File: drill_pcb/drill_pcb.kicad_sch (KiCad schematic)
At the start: 38 parts, among them SW1 RPi reset, U1 PCA9306, U2 Pico, U3 L7805, U4 IFX007T, U5 IFX007T, U6 ACS712xLCTR-20A

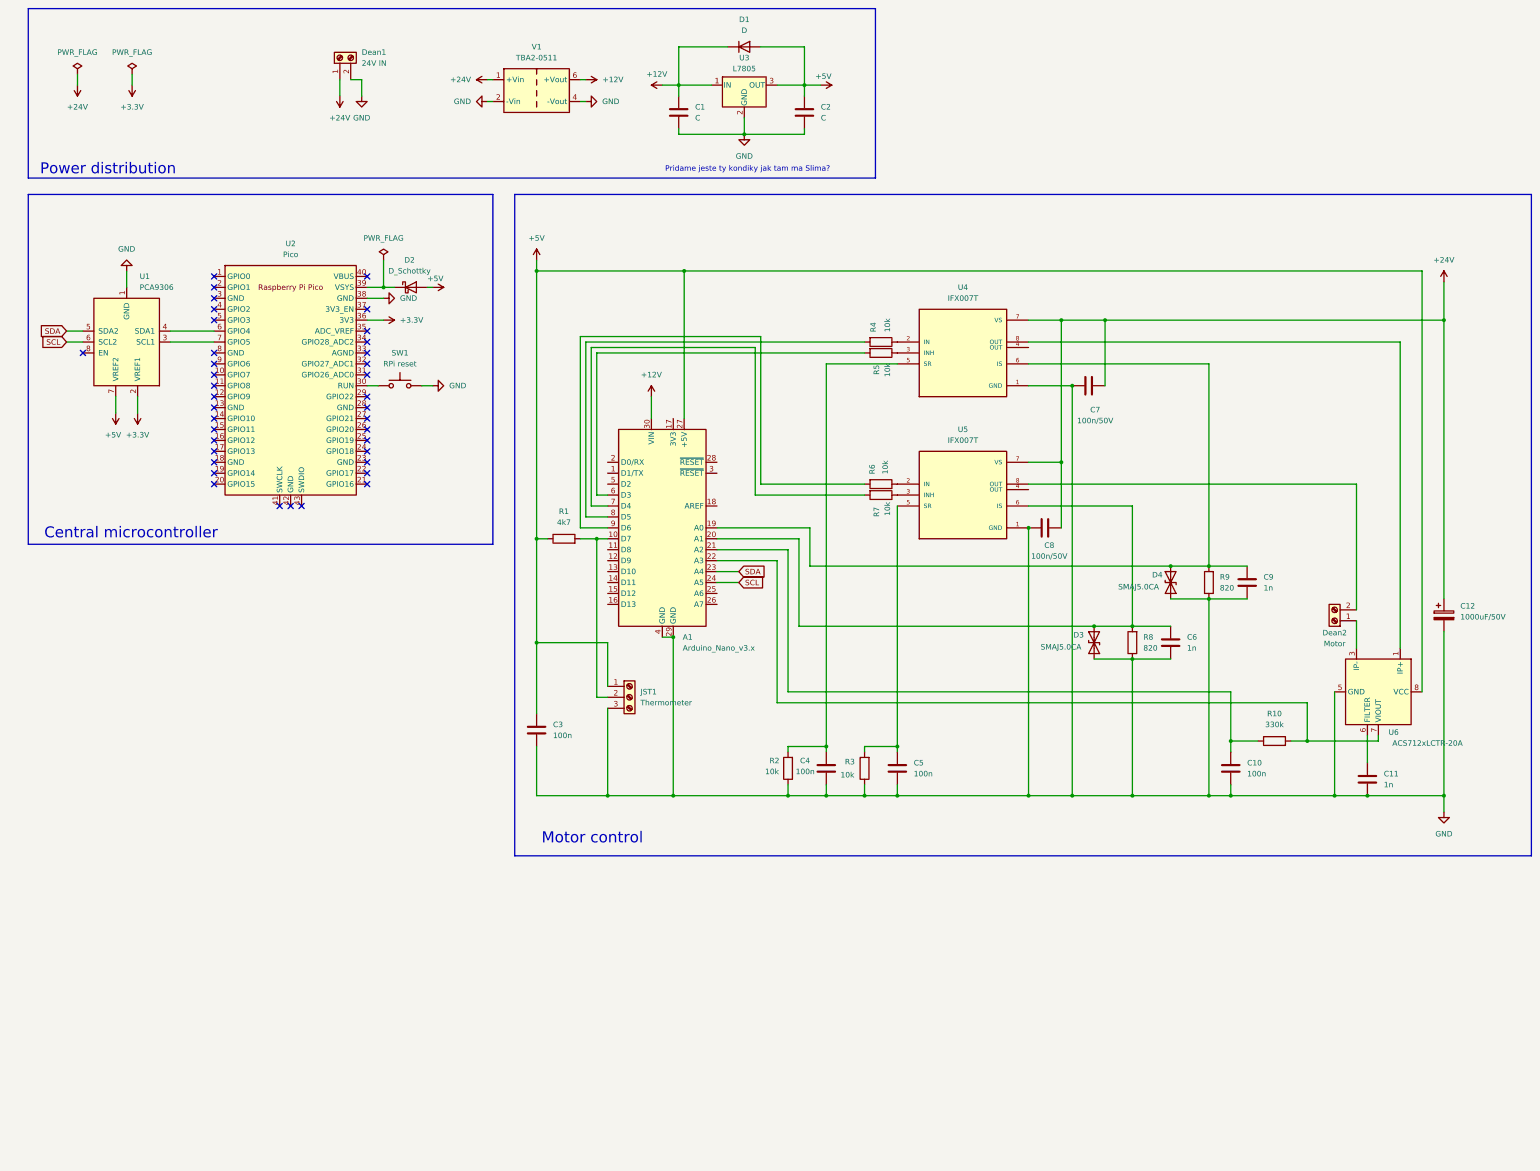
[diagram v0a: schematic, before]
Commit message: Library manager update
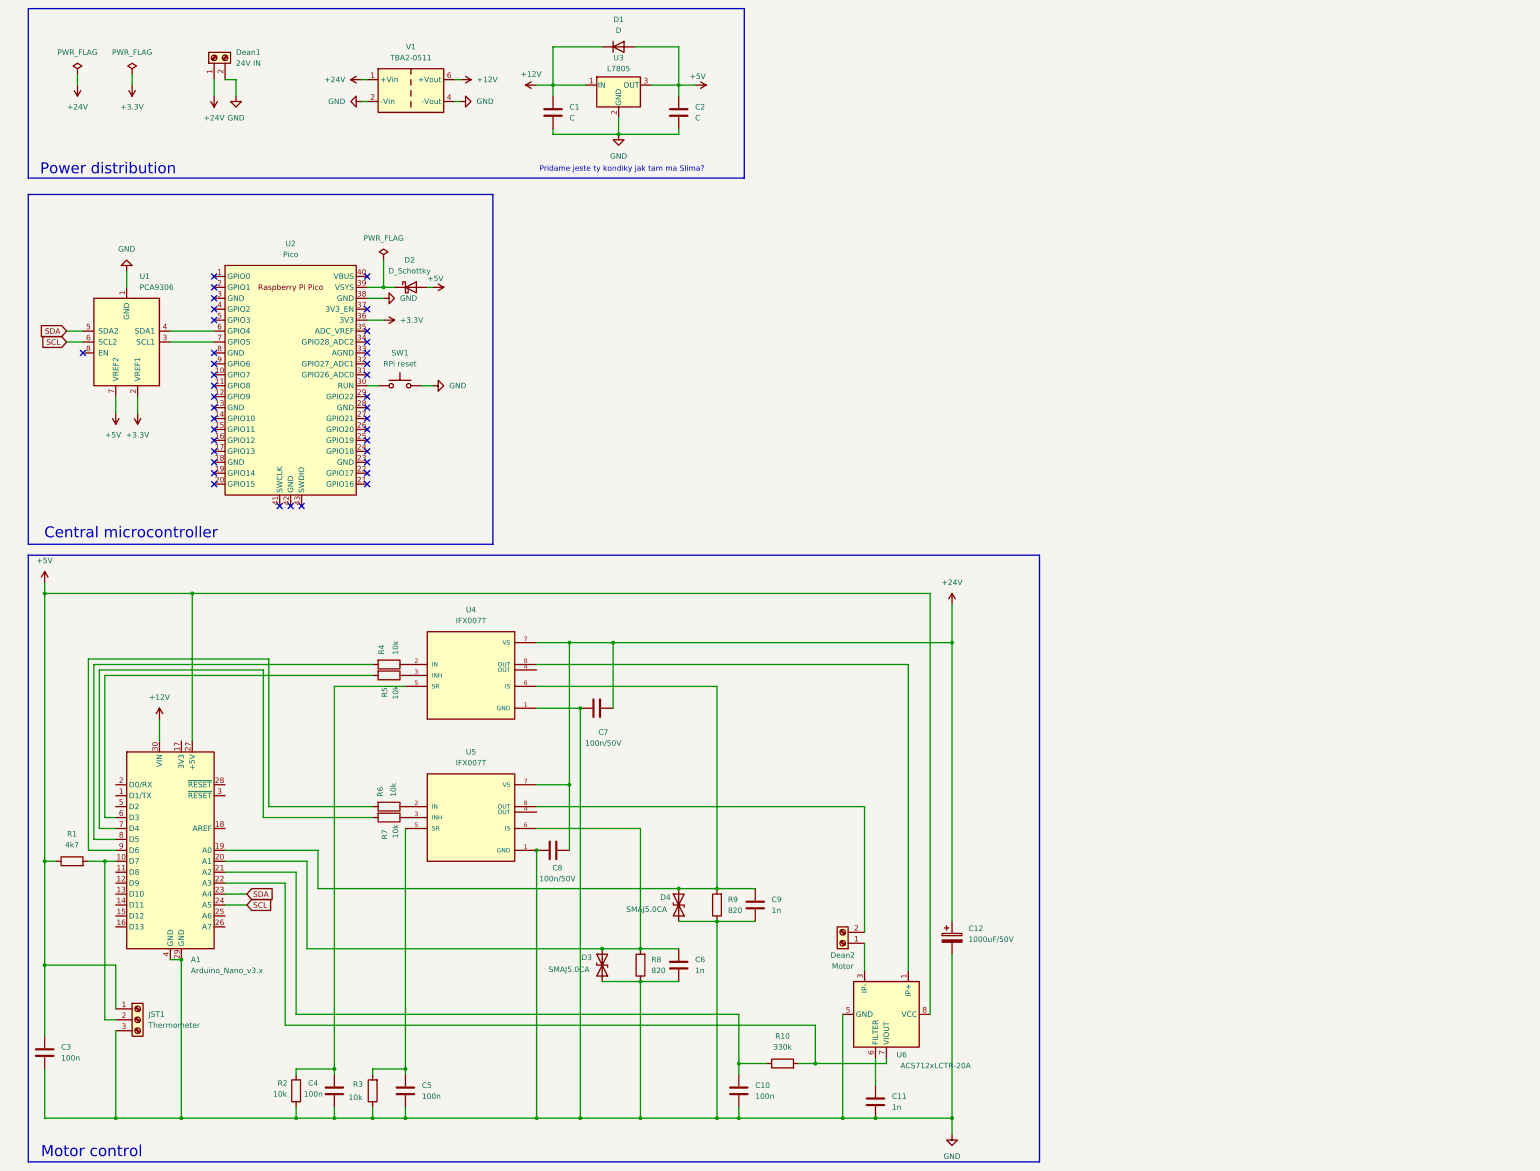
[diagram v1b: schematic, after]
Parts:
- U1: footprint i2c_levl:i2c_levl_shifter -> drill_i2c_level_shifter:i2c_levl_shifter
- U2: footprint MCU_RaspberryPi_and_Boards:RPi_Pico_SMD_TH -> drill_RP-Pico Libraries:RPi_Pico_SMD_TH
- V1: footprint i2c_levl:dcdc_menic -> drill_dcdc_converter_LM2596:dcdc_menic
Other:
- moved on the sheet: A1, C1, C10, C11, C12, C2, C3, C4, C5, C6, C7, C8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
